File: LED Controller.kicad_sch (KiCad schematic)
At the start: 18 parts, among them J1 Conn_01x03, J2 Conn_01x03, J3 Conn_01x03, J4 Conn_01x03, J5 Conn_01x03, J6 12v IN, J7 SPI, J8 Conn_01x02, U1 4504, U2 L7805

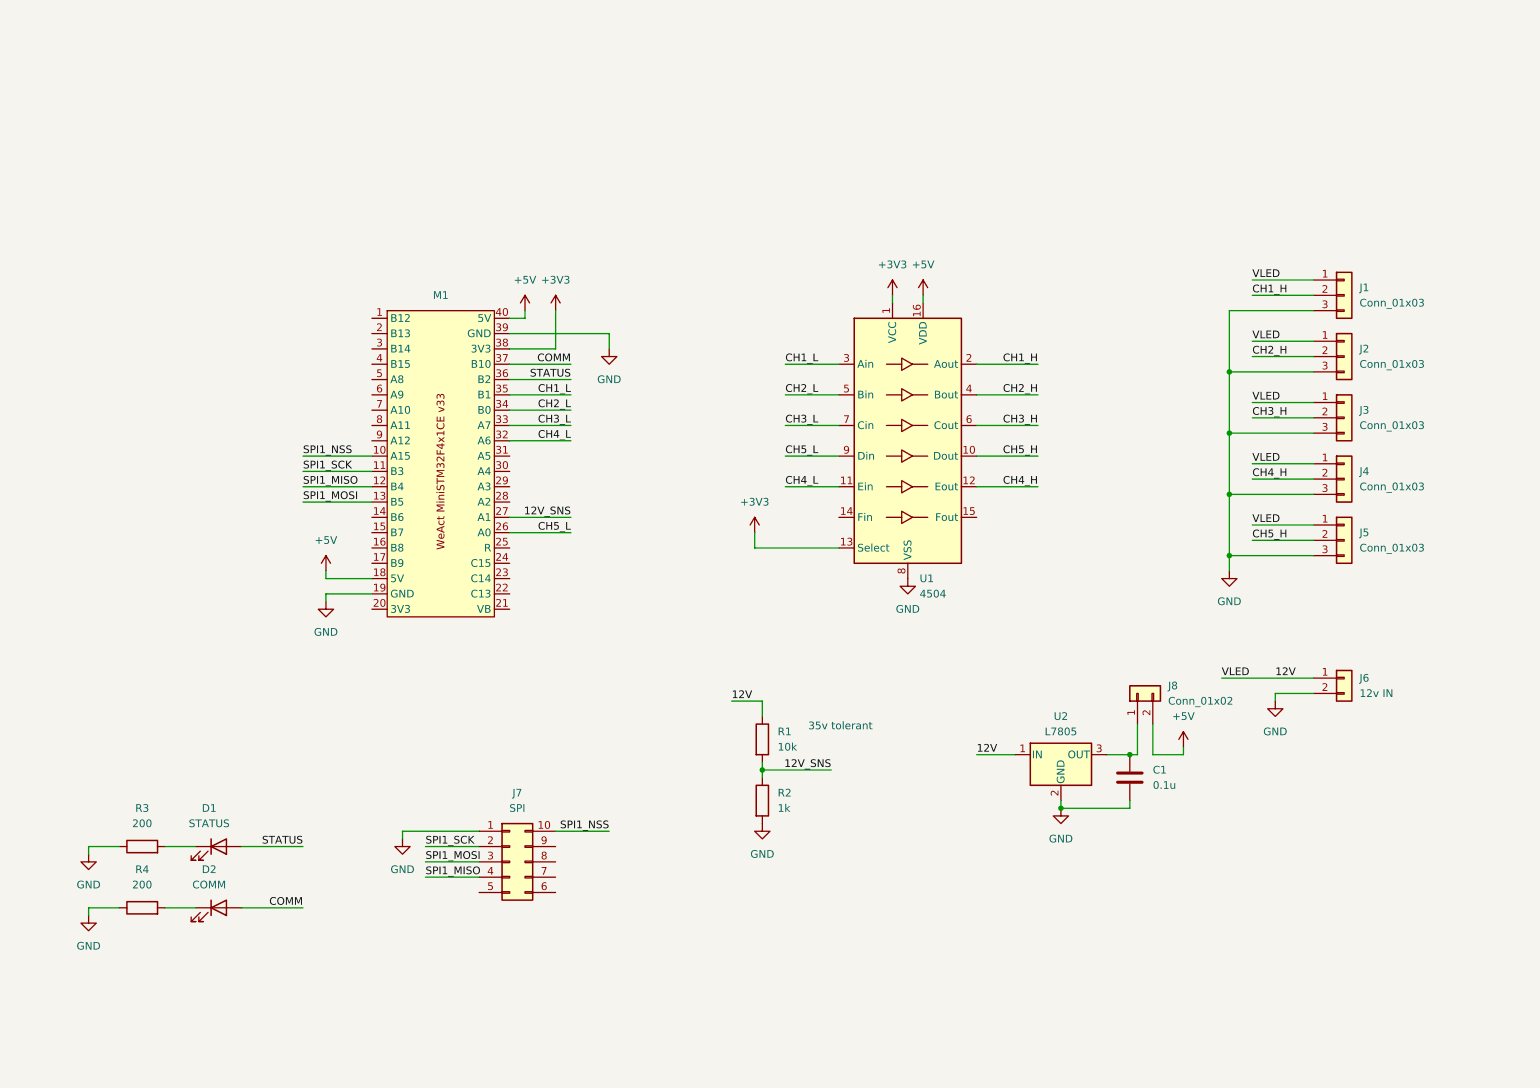
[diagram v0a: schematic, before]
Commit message: Add export
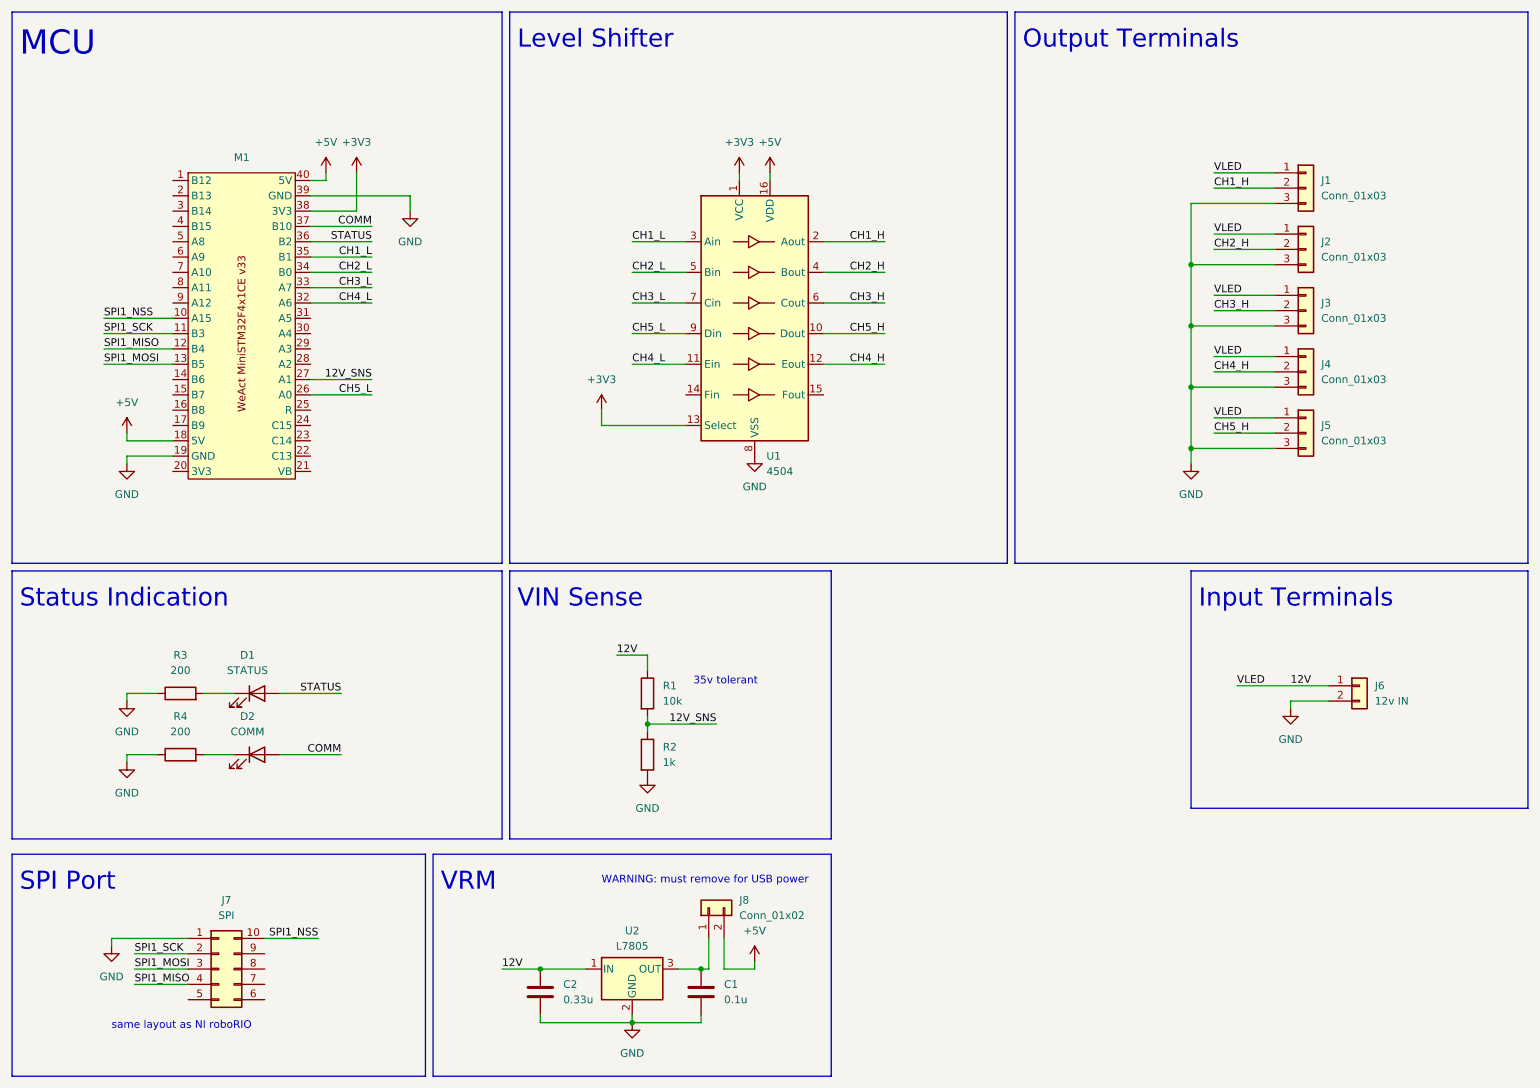
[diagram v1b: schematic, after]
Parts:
- added C2: 0.33u, Capacitor_THT:CP_Radial_D4.0mm_P1.50mm, symbol Device:C
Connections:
- net 12V: now also C2.1
- net GND: now also C2.2
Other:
- note added: "Input Terminals"
- note added: "Level Shifter"
- note added: "MCU"
- note added: "Output Terminals"
- note added: "SPI Port"
- note added: "Status Indication"
- note added: "VIN Sense"
- note added: "VRM"
- note added: "WARNING: must remove for USB power"
- note added: "same layout as NI roboRIO"
- moved on the sheet: C1, D1, D2, J1, J2, J3, J4, J5, J6, J7, J8, M1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
